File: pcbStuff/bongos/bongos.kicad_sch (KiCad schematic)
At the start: 42 parts, among them SW1 SW_Push, SW2 SW_Push, SW3 SW_Push, SW4 SW_Push, SW5 SW_Push, U1 74LS04, U10 74LS04, U11 74LS74, U12 74LS74, U13 LM555xN, U14 74LS32, U15 74LS32, U16 LM555xN, U17 74LS32, U2 74LS04, U3 74LS08, U4 74LS74, U5 74LS74, U6 74LS08, U7 74LS00, U8 74LS32, U9 74LS74

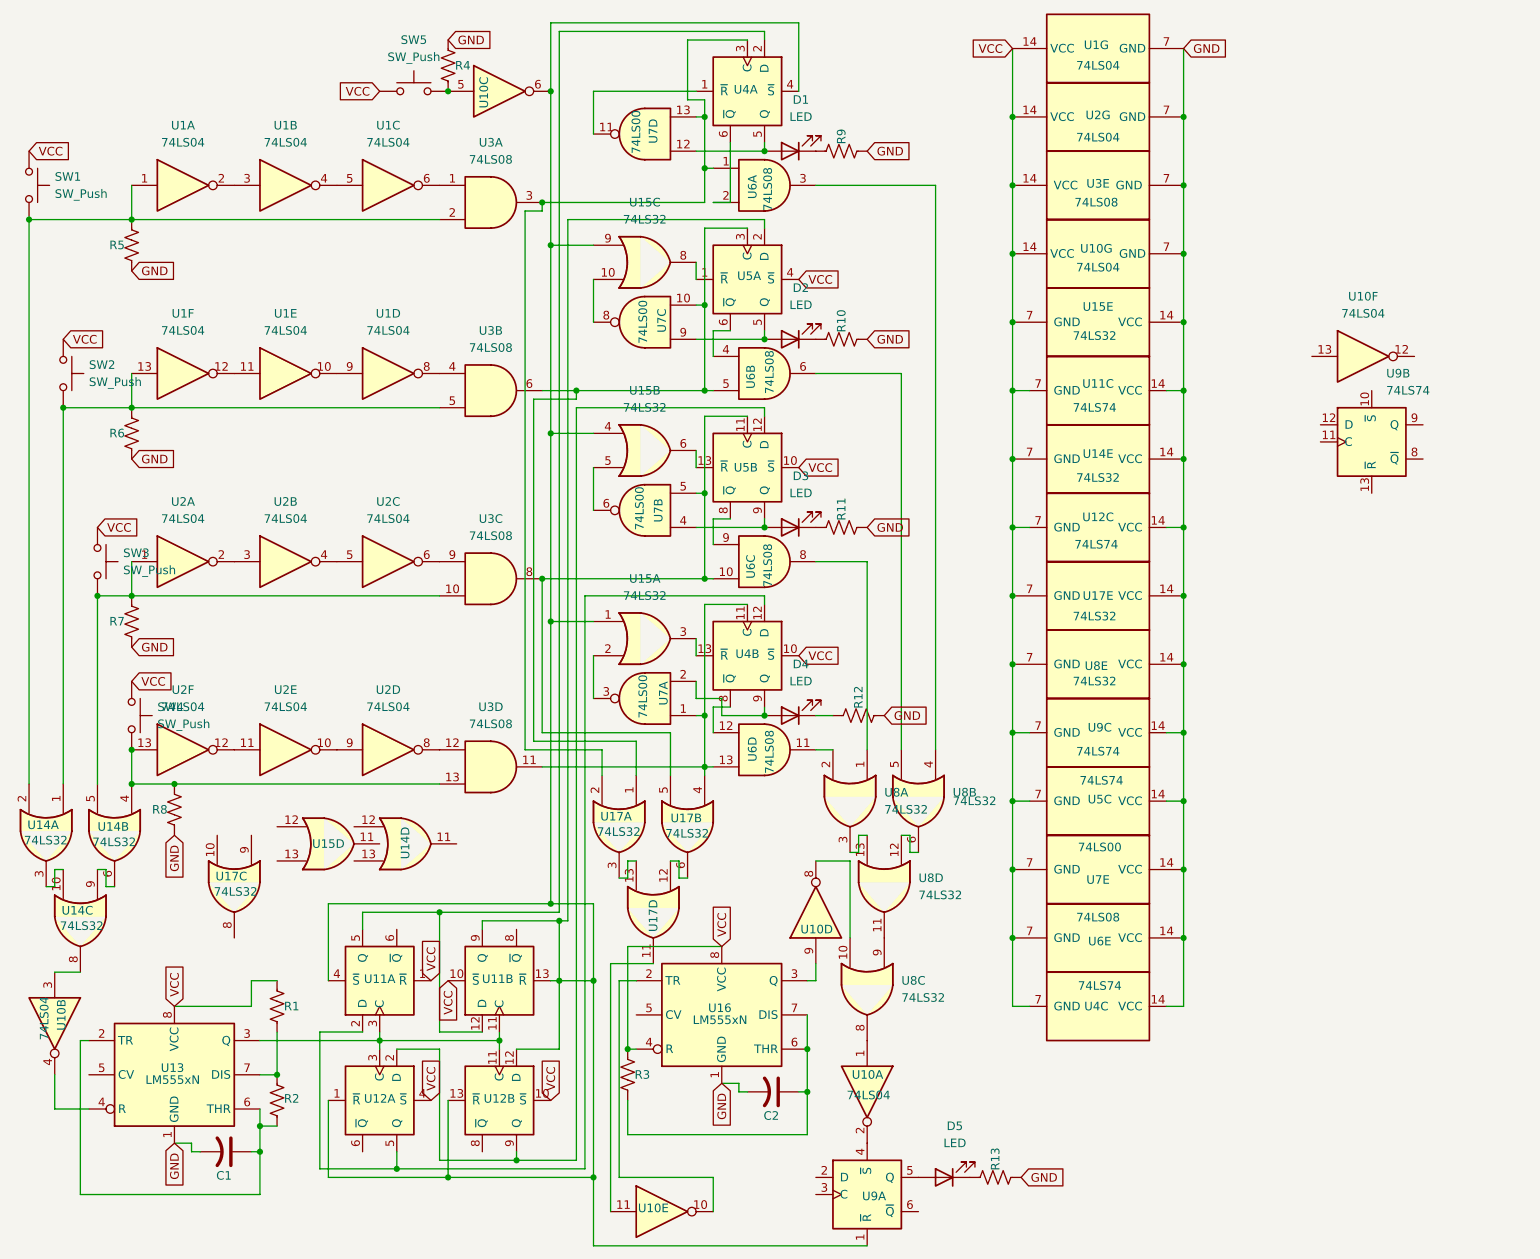
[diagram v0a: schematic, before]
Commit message: fable foo
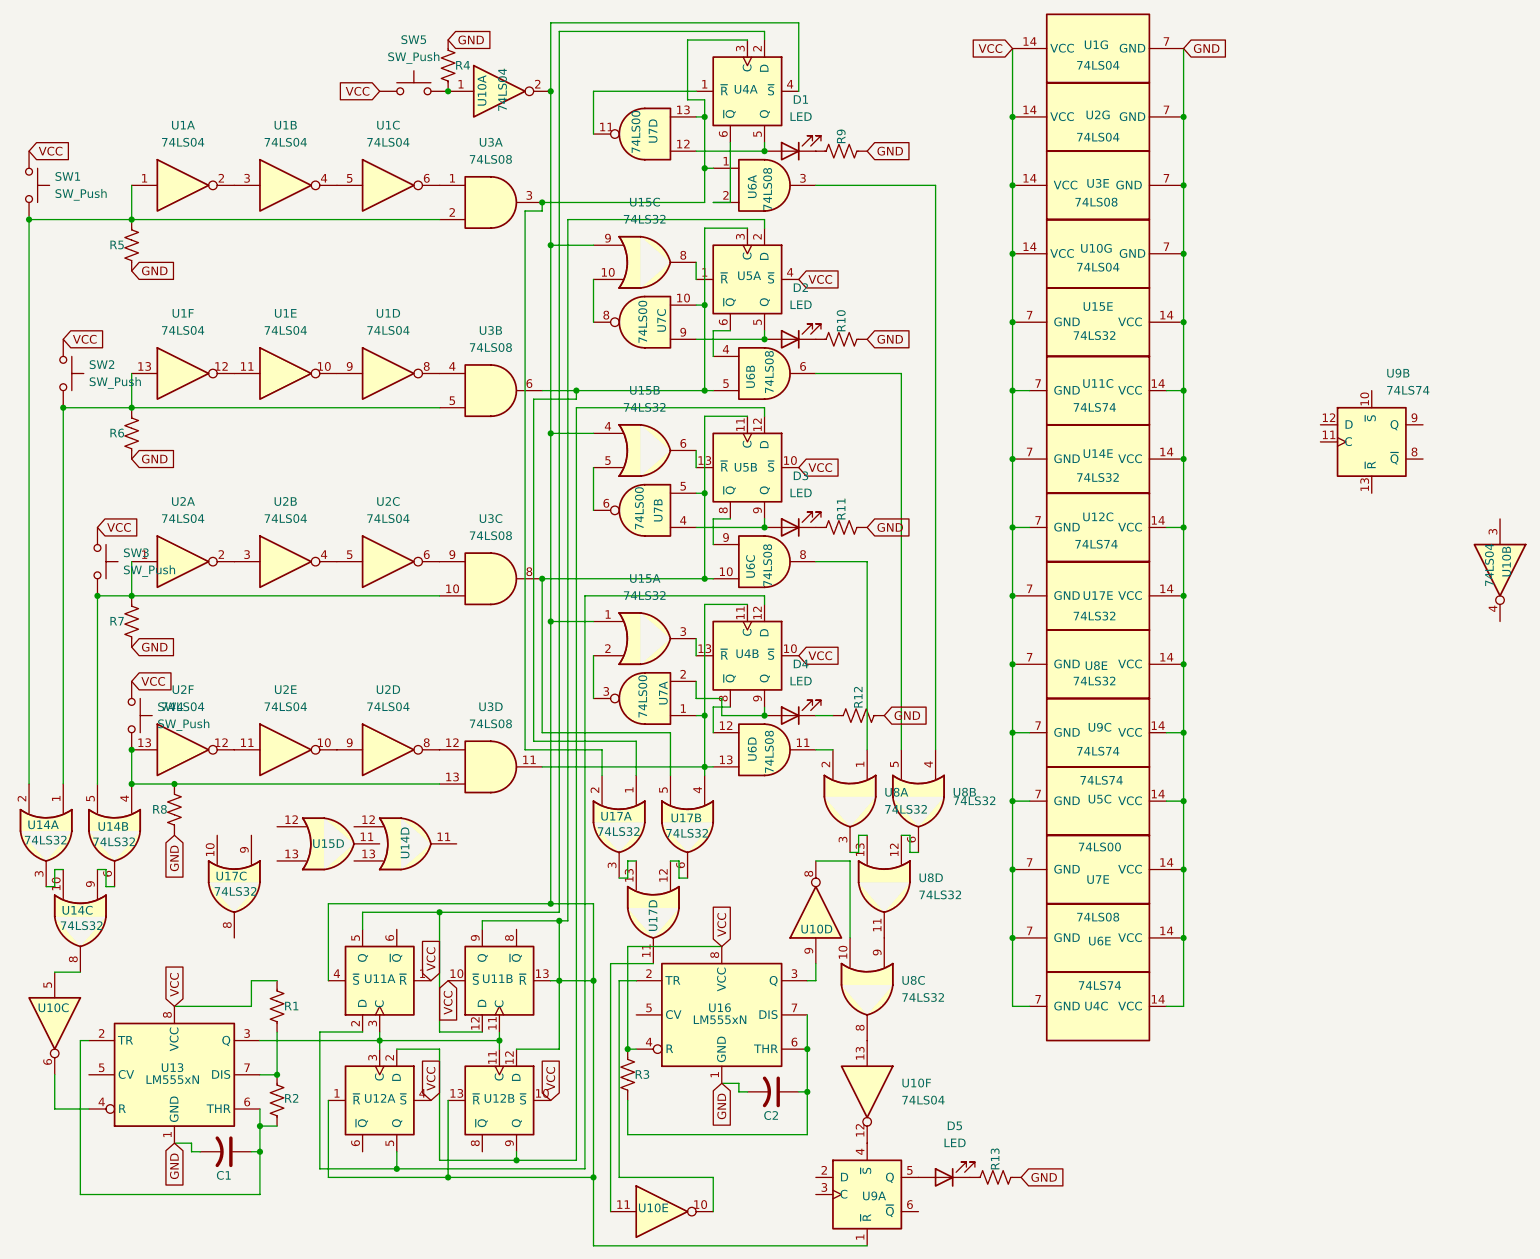
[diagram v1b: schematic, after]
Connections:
- net at R4.2, SW5.2: now also U10.1; no longer U10.5
- net at U11.13 (~{R}), U11.4 (~{S}), U11.9 (Q)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: now also U10.2; no longer U10.6
- net at U9.4 (~{S}): now also U10.12; no longer U10.2
- net at U10.13: now also U8.8
- net at U10.3: no longer U14.8
- net at U10.4: no longer U13.4 (R)
- new net: U10.6, U13.4 (R)
- new net: U10.5, U14.8
